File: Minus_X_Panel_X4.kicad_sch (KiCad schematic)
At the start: 1 part, among them J1 SM05B-SRSS-TB_LF__SN_

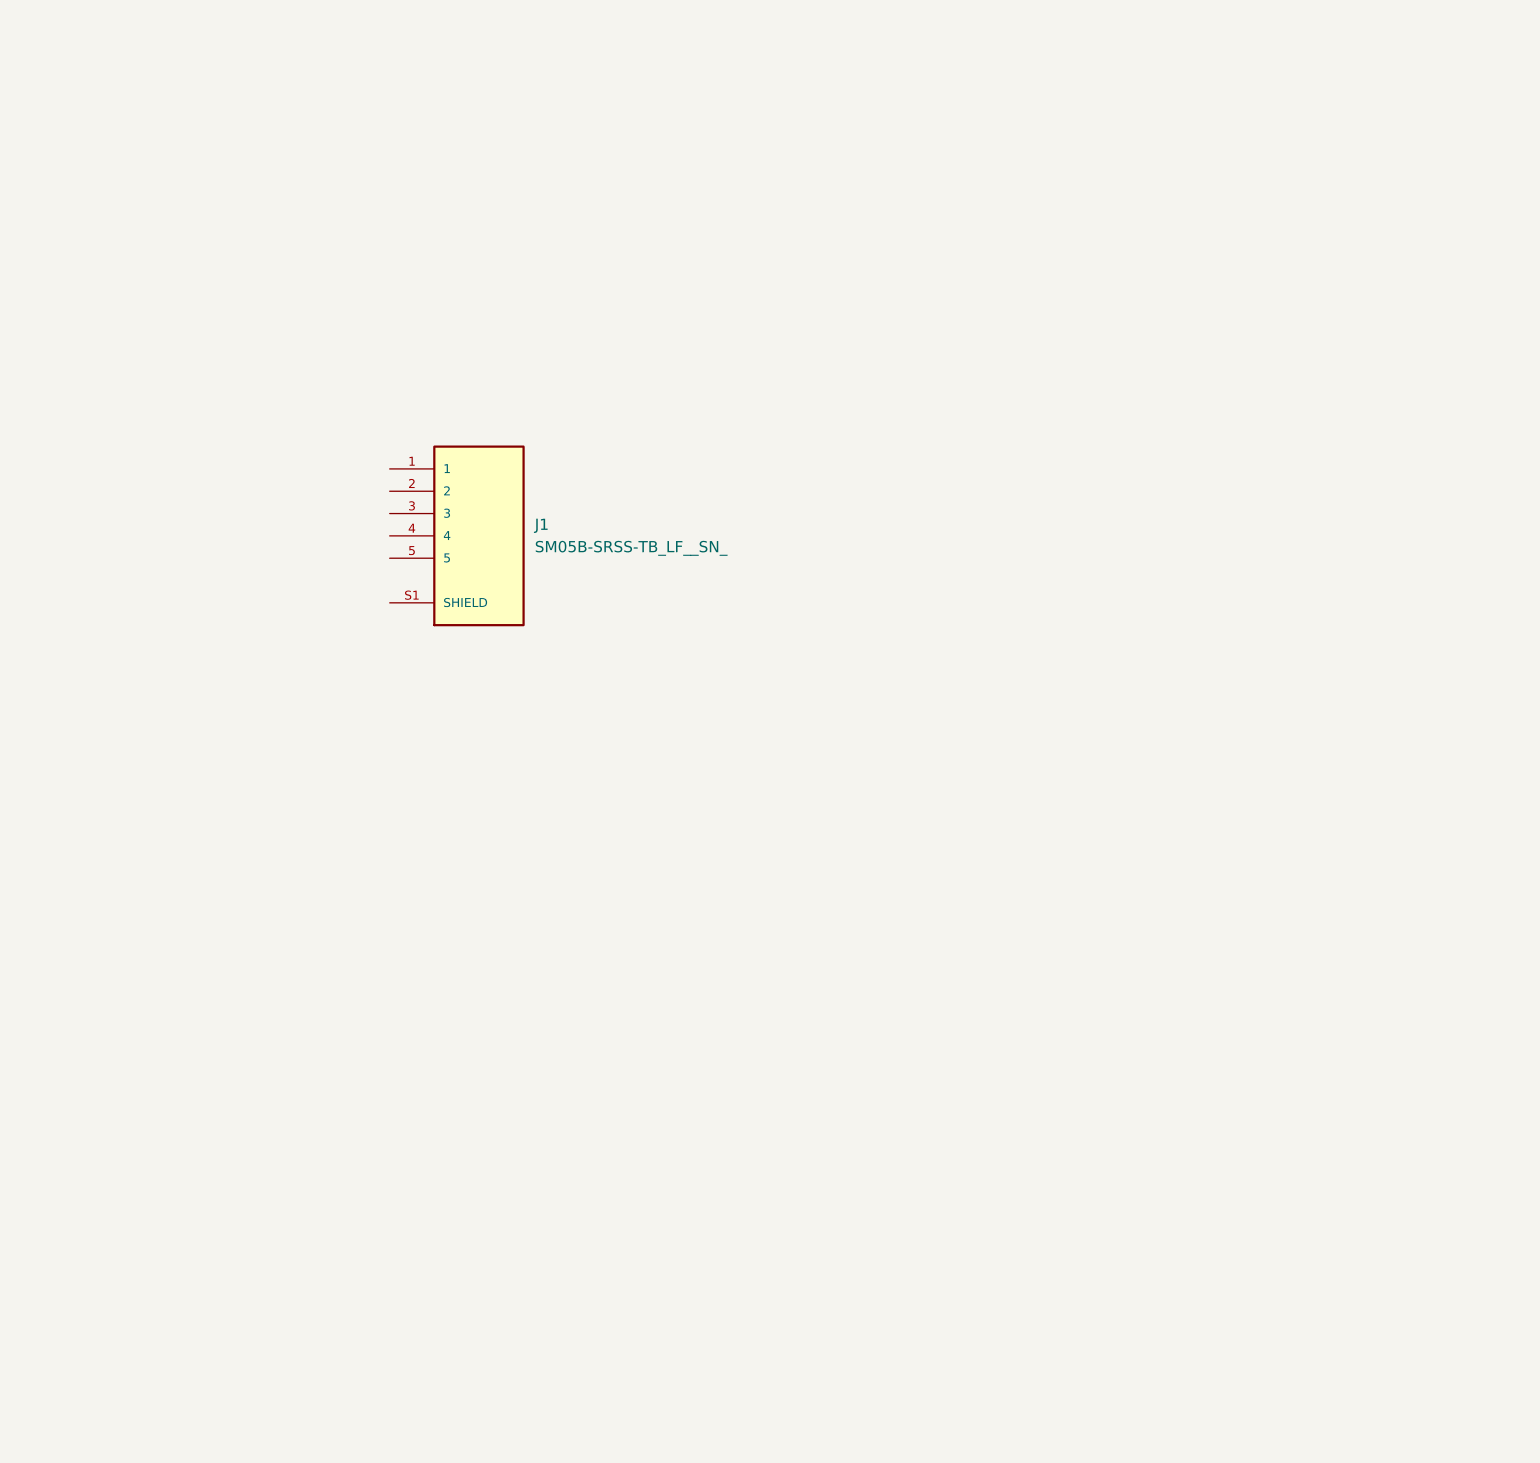
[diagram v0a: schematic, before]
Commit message: Symbol and foot print id almost ready
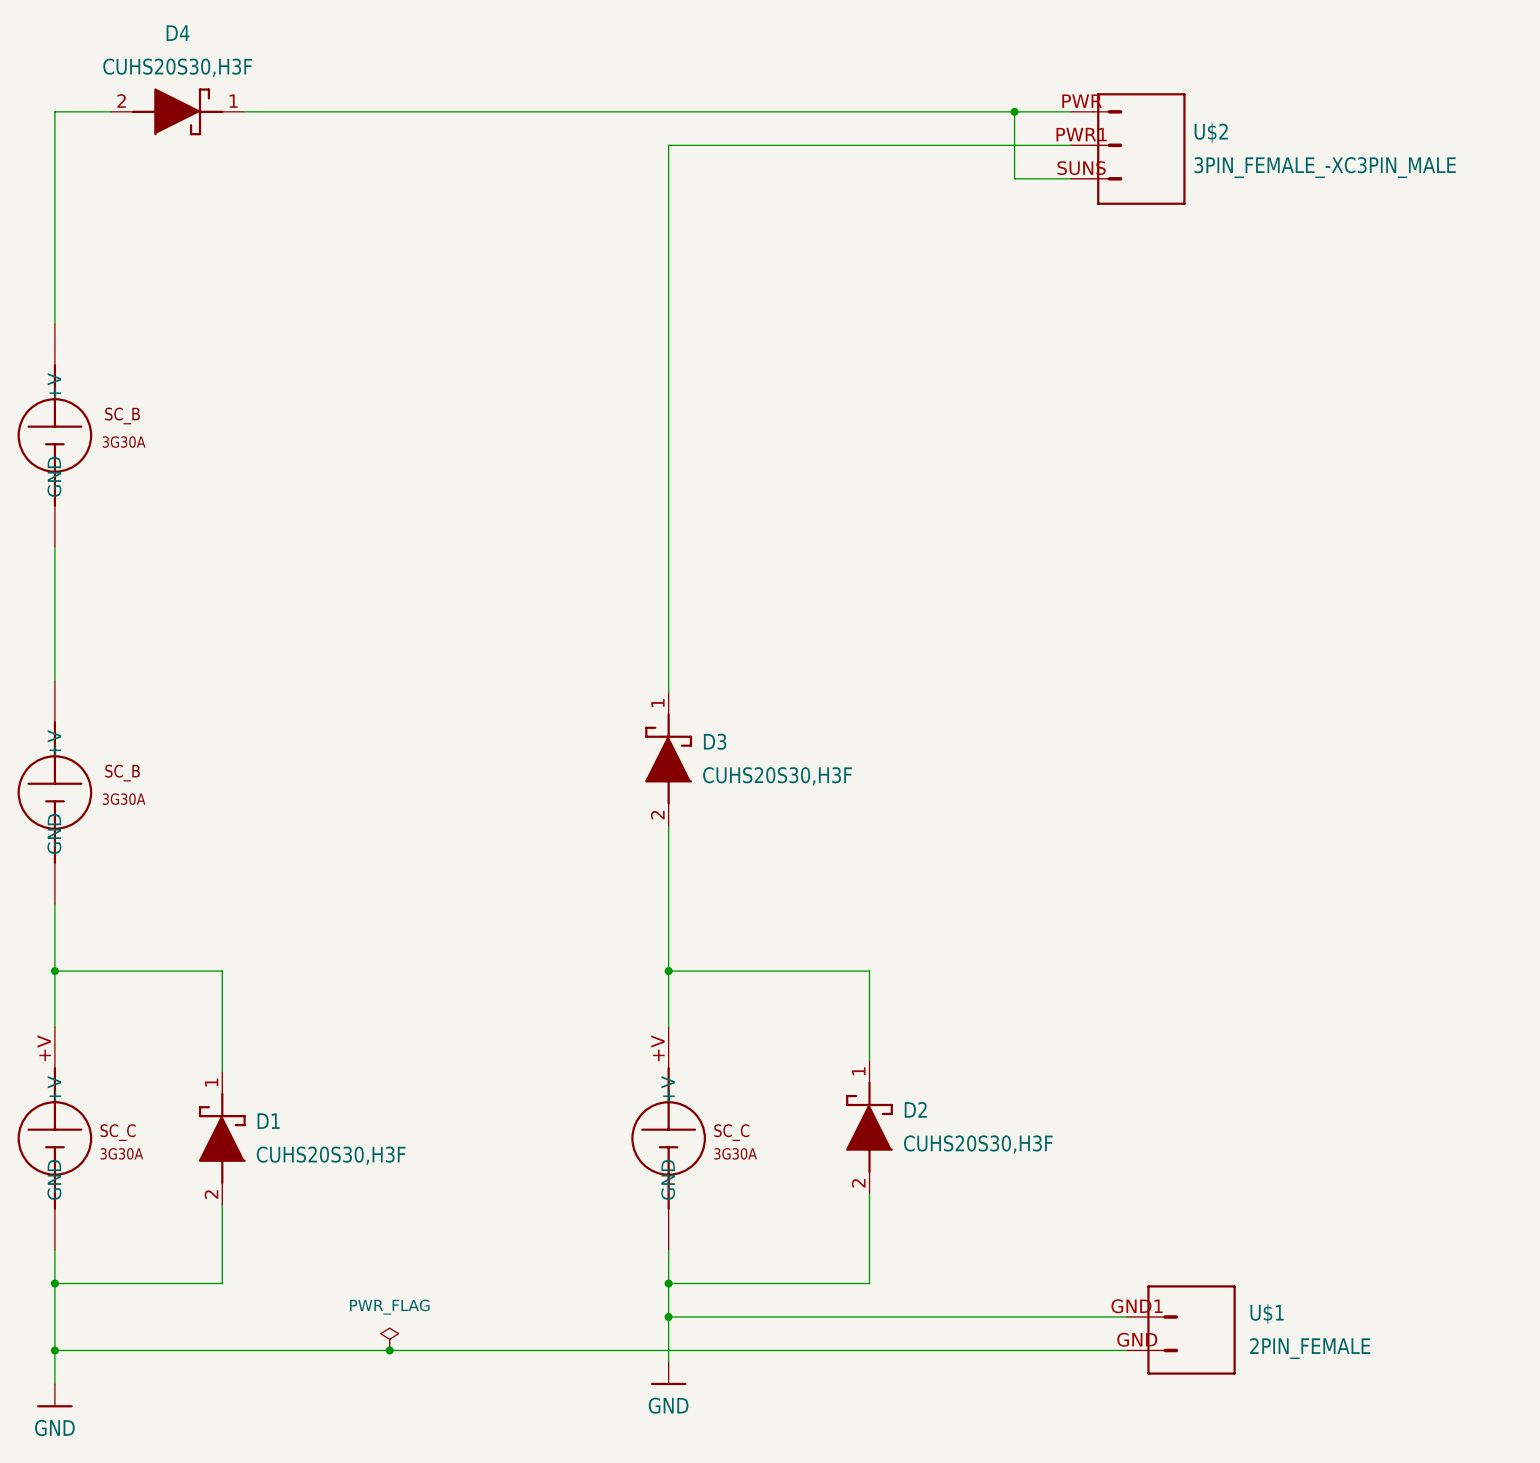
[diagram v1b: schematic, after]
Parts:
- removed J1: SM05B-SRSS-TB_LF__SN_, Custom-Footprints:JST_SM05B-SRSS-TB_LF__SN_, symbol Custom-Symbols:SM05B-SRSS-TB_LF__SN_
- added D1, D2, D3, D4: CUHS20S30,H3F, Custom-Footprints:CUHS20S30,H3F, symbol Custom-Symbols:CUHS20S30,H3F
- added S1, S4: solar_cell_B, Custom-Footprints:solar_cell_B, symbol Custom-Symbols:solar_cell_B
- added S2, S3: Solar_cell_C, Custom-Footprints:solar_cell_C, symbol Custom-Symbols:Solar_cell_C
- added U$1: 2PIN_FEMALE, Custom-Footprints:FSR-41057-02-F, symbol Custom-Symbols:2PIN_FEMALE
- added U$2: 3PIN_FEMALE_-XC3PIN_MALE, Custom-Footprints:FSR-41057-03-F, symbol Custom-Symbols:3PIN_FEMALE_-XC3PIN_MALE
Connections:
- new net: D4.2 (A), S1.+V
- new net: S1.GND, S4.+V
- new net: D4.1 (K), U$2.PWR, U$2.SUNS
- new net: D3.1 (K), U$2.PWR1
- new net: D2.1 (K), D3.2 (A), S3.+V
- new net: D1.1 (K), S2.+V, S4.GND
- new net GND: D1.2 (A), D2.2 (A), S2.GND, S3.GND, U$1.GND, U$1.GND1
